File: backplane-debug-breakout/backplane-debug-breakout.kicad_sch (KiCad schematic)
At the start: 16 parts, among them J1 Conn_02x08_Odd_Even, J2 Conn_01x04, J4 Conn_01x02_Socket, J5 Conn_01x04, J6 629105150521, SW1 SW_Push_DPDT, SW2 SW_Omron_B3FS, SW3 EG1218, U1 UMFT234XF

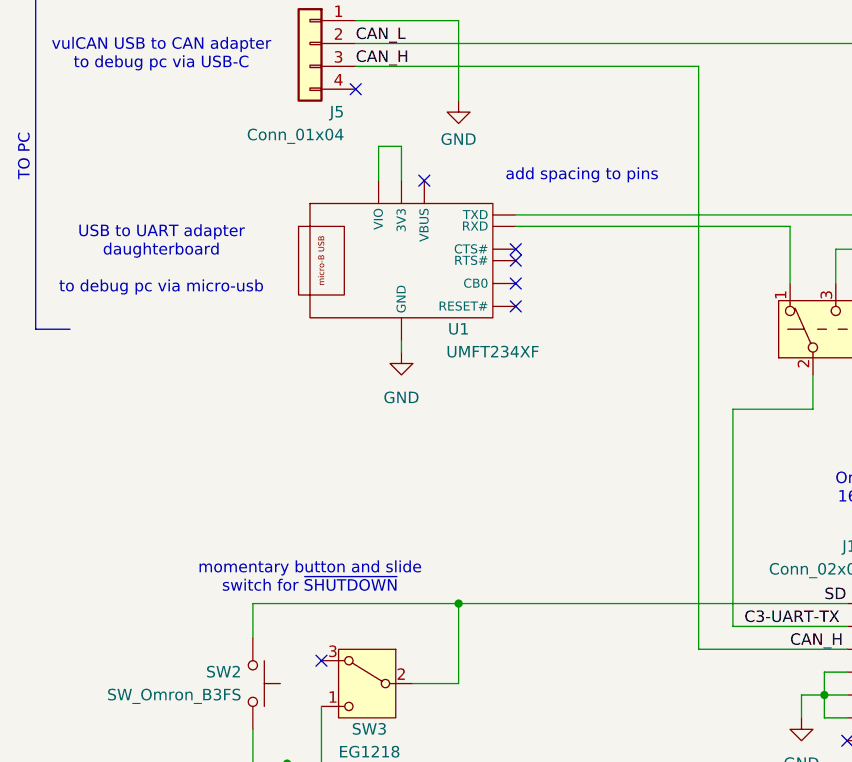
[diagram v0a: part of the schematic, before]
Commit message: finished schematic, updated pcb
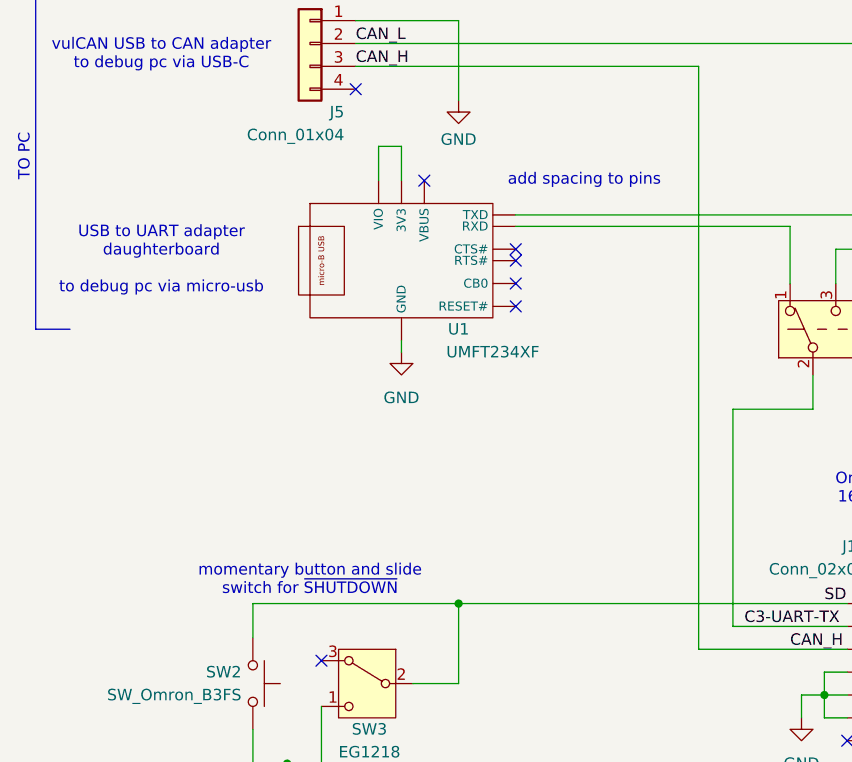
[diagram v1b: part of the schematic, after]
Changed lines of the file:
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@@
 	(text "momentary button and slide \nswitch for ~{SHUTDOWN}"
 		(exclude_from_sim no)
-		(at 80.01 87.376 0)
+		(at 80.01 87.63 0)
 		(effects
 			(font
@@
 	(text "add spacing to pins"
 		(exclude_from_sim no)
-		(at 110.236 42.672 0)
+		(at 110.49 43.18 0)
 		(effects
 			(font
